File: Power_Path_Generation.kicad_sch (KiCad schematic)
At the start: 11 parts, among them Q701 PMOS SI2365EDS-T1-GE3, U701 TPS3839G33DQNR, U702 TPS7A0233DQNR

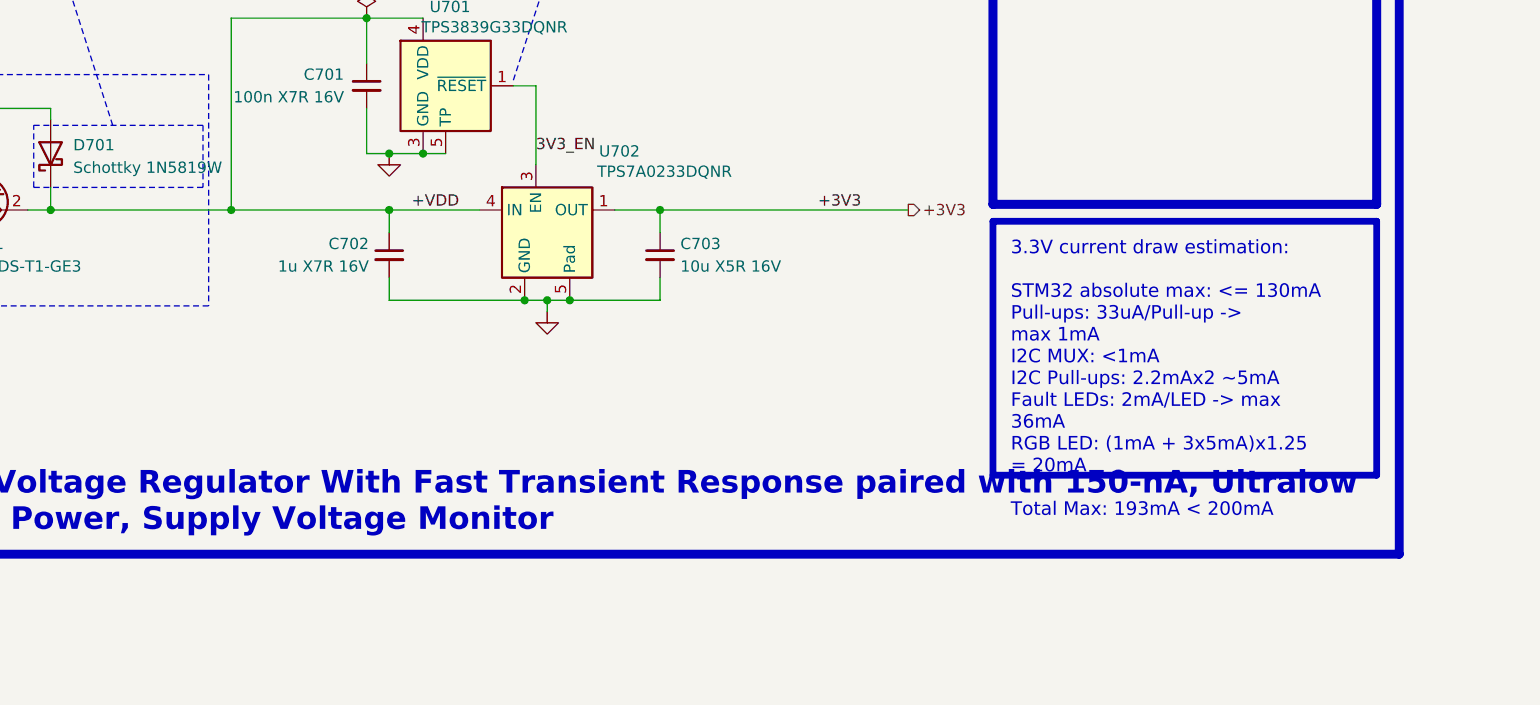
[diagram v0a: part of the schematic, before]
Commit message: Advanced rough layout
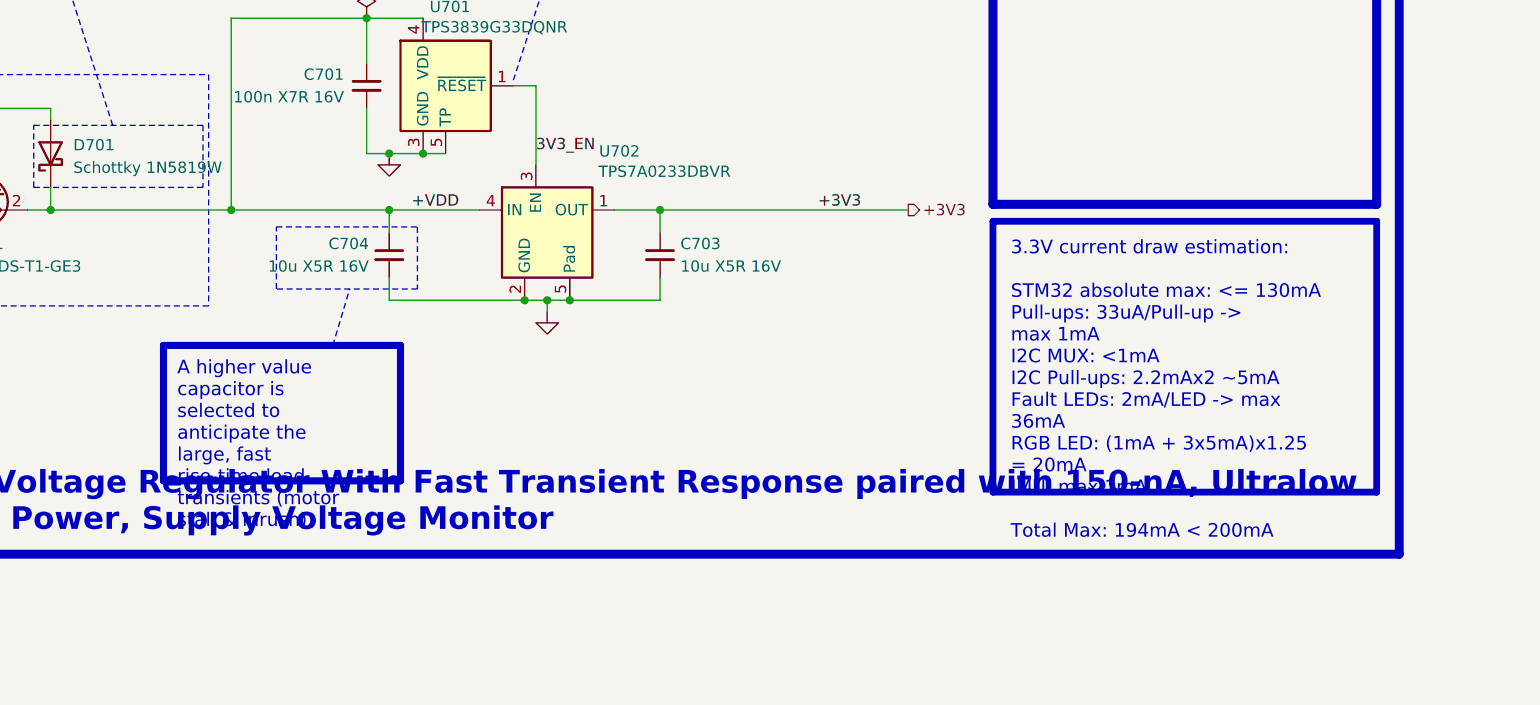
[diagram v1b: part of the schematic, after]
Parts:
- removed C702: 1u X7R 16V, Capacitor_SMD:C_0603_1608Metric, symbol Device:C_Small
- added C704: 10u X5R 16V, Capacitor_SMD:C_0603_1608Metric, symbol Device:C_Small
- U702: value TPS7A0233DQNR -> TPS7A0233DBVR; footprint Package_SON:Texas_X2SON-4_1x1mm_P0.65mm -> Package_TO_SOT_SMD:SOT-23-5; symbol 0_Plume:TPS7A20xxxDQN -> 0_Plume:TPS7A20xxxDBVR; Manufacturer Part Number TPS7A0233DQNR -> TPS7A0233DBVR; Supplier Part Number 595-TPS7A0233DQNR -> 595-TPS7A0233DBVR
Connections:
- net +VDD: now also C704.1
- net GND: now also C704.2
